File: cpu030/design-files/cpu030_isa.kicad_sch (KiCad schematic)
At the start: 15 parts, among them J401 ISACTL JTAG, U401 ATF1508AS, U402 MC74ACT05DG

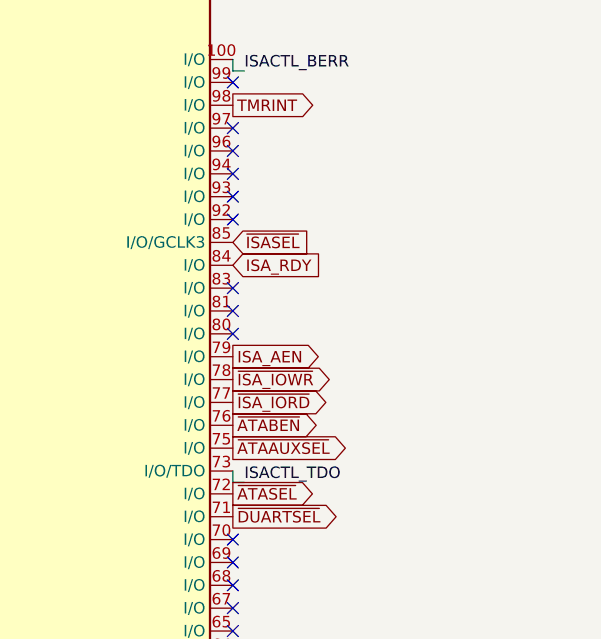
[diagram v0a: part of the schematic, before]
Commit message: Checkpoint -- expansion interface and PSU placeholders.  More work to do, but I want to get mounting holes placed.
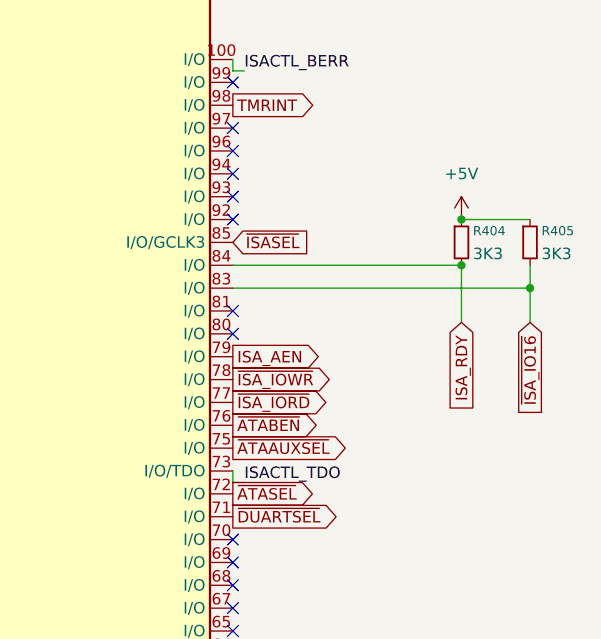
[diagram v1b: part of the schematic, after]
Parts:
- added R404, R405: 3K3, Resistor_SMD:R_0805_2012Metric, symbol Device:R_Small
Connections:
- net +5V: now also R404.1, R405.1
- net ISA_RDY: now also R404.2
- net ~{ISA_IO16}: now reaches U401.83 (I/O)
- net ~{ISA_IO16}: now also R405.2
- no-connect marks 47 -> 46
